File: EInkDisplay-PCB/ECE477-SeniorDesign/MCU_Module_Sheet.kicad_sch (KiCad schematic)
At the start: 43 parts, among them J1 Conn_01x05, J2 Conn_01x05_Pin, U1 PTS526 SK15 SMTR2 LFS, U2 STM32L496ZGTxP, Y1 Y1

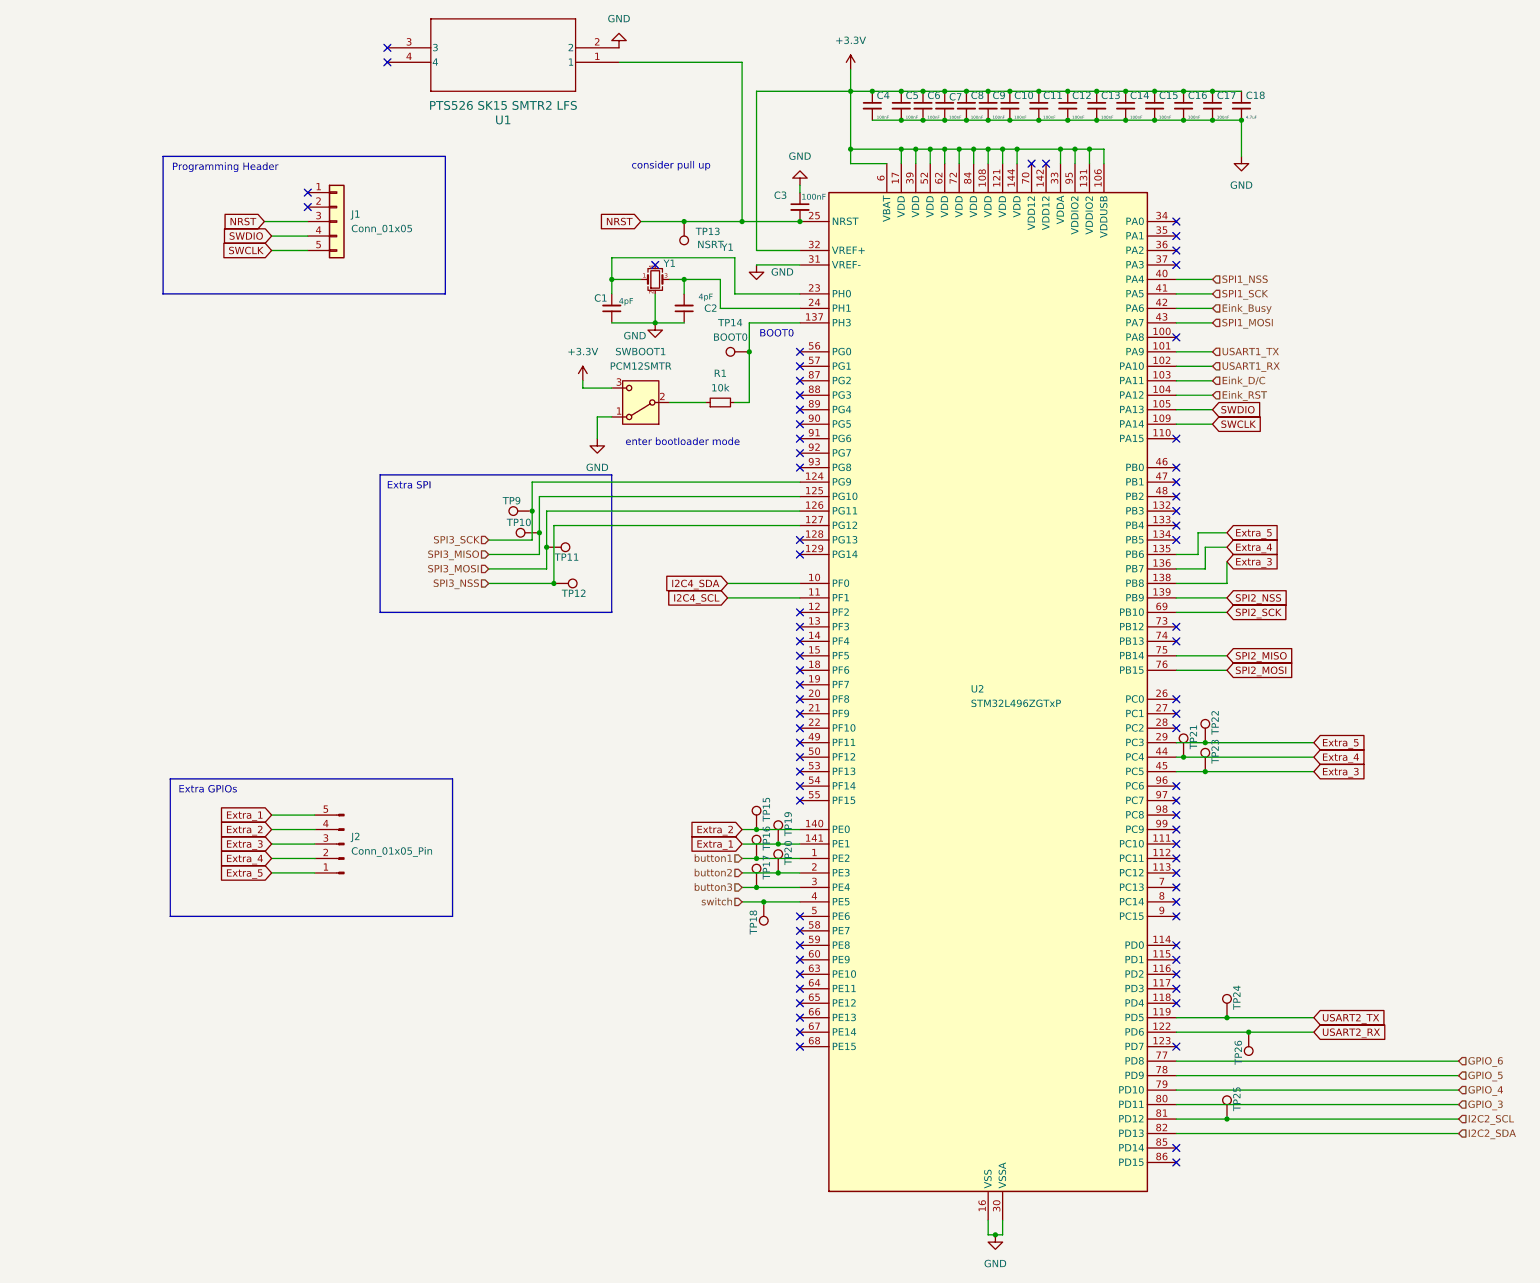
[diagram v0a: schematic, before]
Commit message: pushing
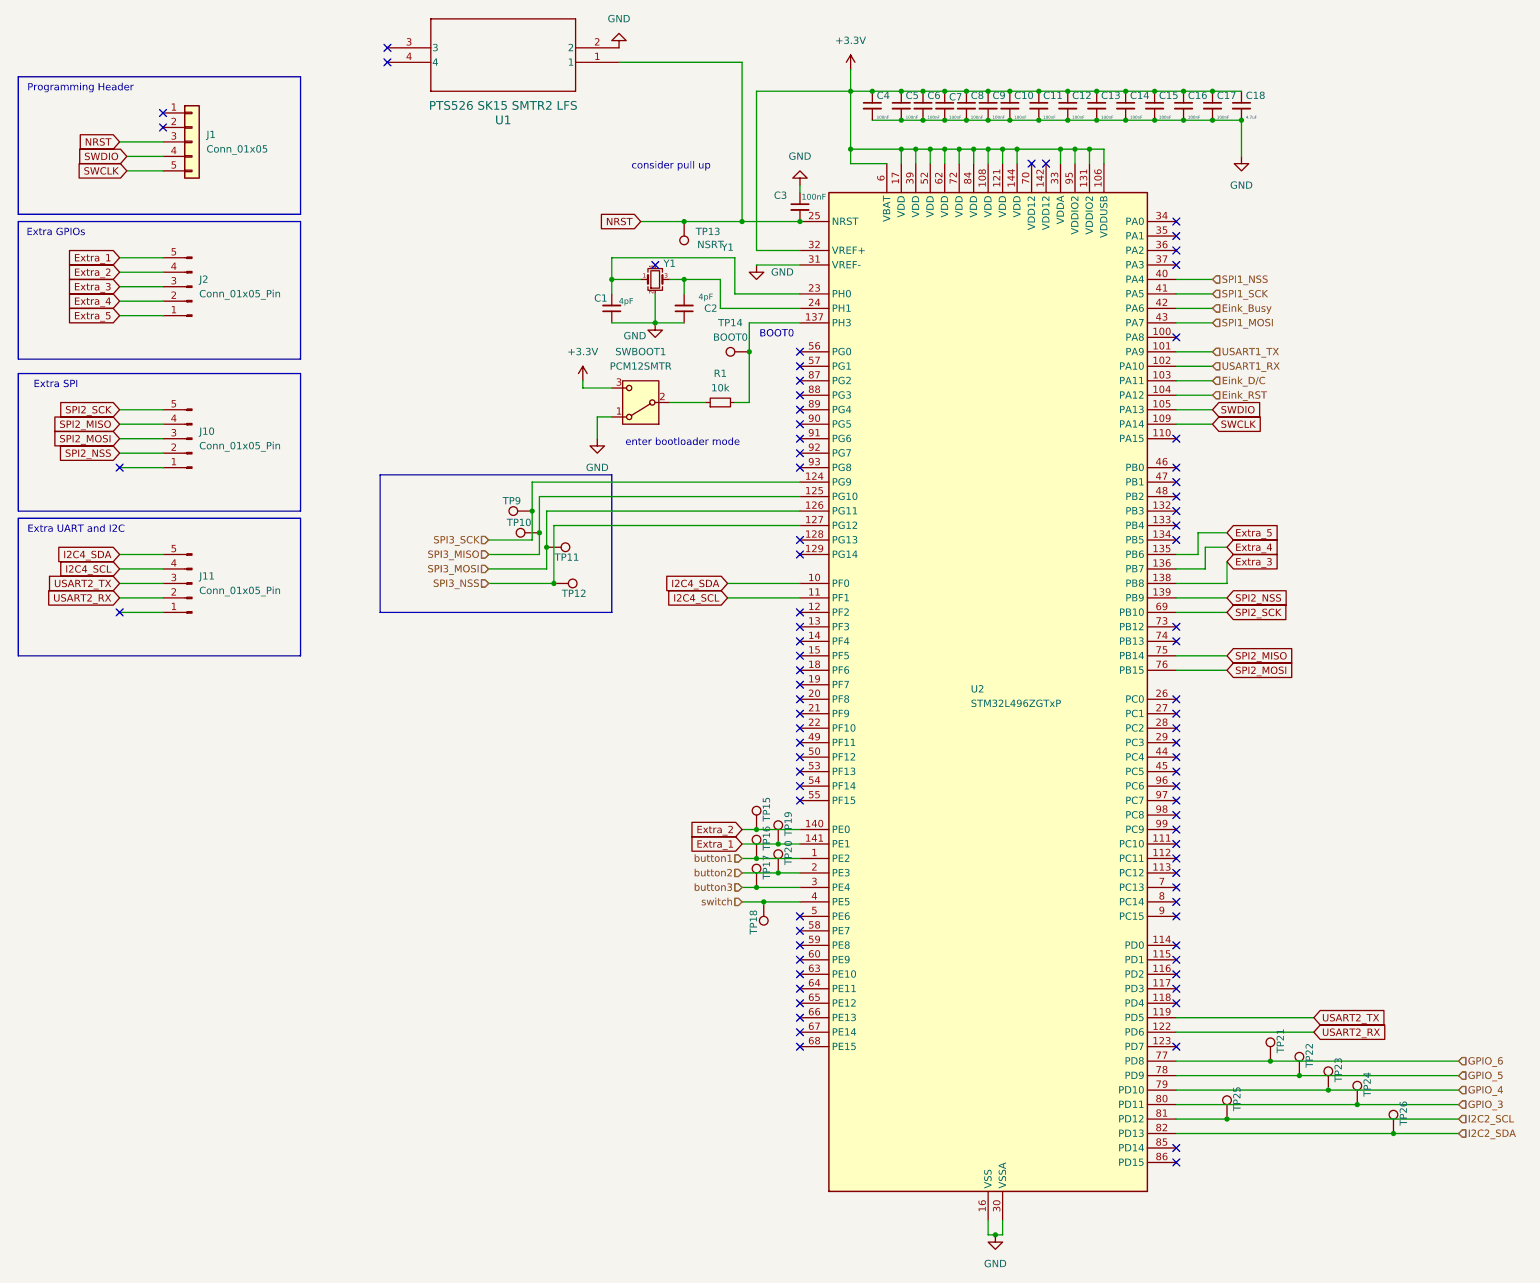
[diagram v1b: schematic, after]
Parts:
- added J10, J11: Conn_01x05_Pin, Connector_PinHeader_1.00mm:PinHeader_1x05_P1.00mm_Vertical, symbol Connector:Conn_01x05_Pin
- SWBOOT1: footprint PCB_Lib:PCM12SMTR_CNK -> Button_Switch_SMD:SW_SPDT_PCM12
- TP10, TP11, TP12, TP13, TP14, TP15, TP16, TP17, TP18, TP19, TP20, TP21, TP22, TP23, TP24, TP25, TP26, TP9: footprint (none) -> TestPoint:TestPoint_Pad_1.0x1.0mm
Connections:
- net Extra_3: no longer TP23.1, U2.45 (PC5)
- net Extra_4: no longer TP21.1, U2.44 (PC4)
- net Extra_5: no longer TP22.1, U2.29 (PC3)
- net GPIO_3: now also TP24.1
- net GPIO_4: now also TP23.1
- net GPIO_5: now also TP22.1
- net GPIO_6: now also TP21.1
- net I2C2_SDA: now also TP26.1
- net I2C4_SCL: now also J11.4 (Pin_4)
- net I2C4_SDA: now also J11.5 (Pin_5)
- net SPI2_MISO: now also J10.4 (Pin_4)
- net SPI2_MOSI: now also J10.3 (Pin_3)
- net SPI2_NSS: now also J10.2 (Pin_2)
- net SPI2_SCK: now also J10.5 (Pin_5)
- net USART2_RX: now also J11.2 (Pin_2); no longer TP26.1
- net USART2_TX: now also J11.3 (Pin_3); no longer TP24.1
- no-connect marks 77 -> 82
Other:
- note added: "Extra UART and I2C"
- moved on the sheet: J1, J2
